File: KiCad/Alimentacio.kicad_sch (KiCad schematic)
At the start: 7 parts, among them J4 Conn_01x01_Pin, U2 LM2596S-5, U7 LM1117DT-3.3

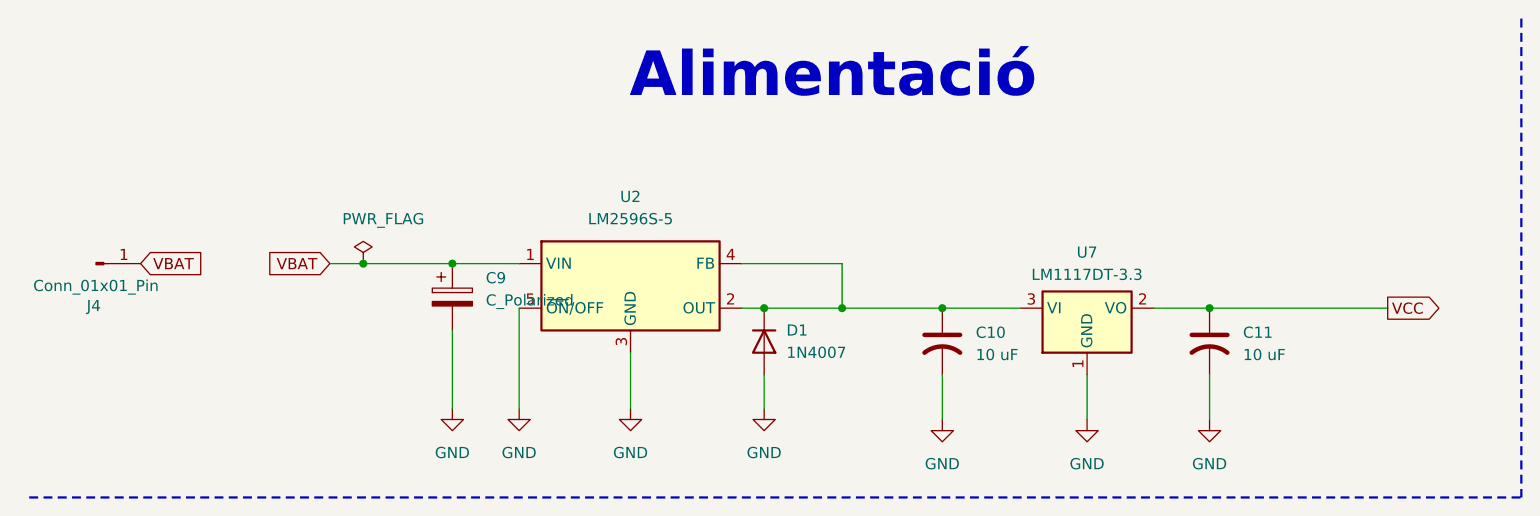
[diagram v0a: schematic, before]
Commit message: Alimentació arreglada
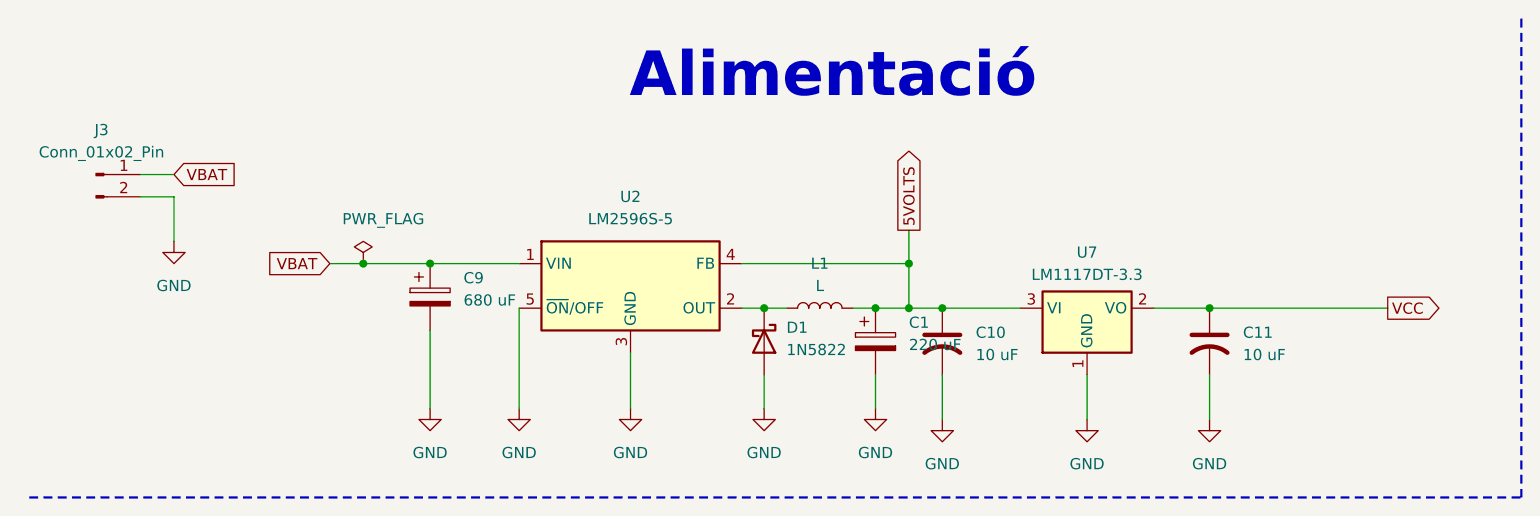
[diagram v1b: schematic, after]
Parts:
- removed D1: 1N4007, Diode_THT:D_DO-41_SOD81_P10.16mm_Horizontal, symbol Diode:1N4007
- removed J4: Conn_01x01_Pin, symbol Connector:Conn_01x01_Pin
- added C1: 220 uF, symbol Device:C_Polarized
- added D1: 1N5822, Diode_THT:D_DO-201AD_P15.24mm_Horizontal, symbol Diode:1N5822
- added J3: Conn_01x02_Pin, symbol Connector:Conn_01x02_Pin
- added L1: L, symbol Device:L
- C9: value C_Polarized -> 680 uF
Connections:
- net GND: now also C1.2, D1.2 (A), J3.2 (Pin_2)
- net VBAT: now also J3.1 (Pin_1)
- net 5VOLTS: now reaches C10.1, U2.4 (FB), U7.3 (VI)
- net 5VOLTS: now also C1.1, L1.2; no longer U2.2 (OUT)
- new net: D1.1 (K), L1.1, U2.2 (OUT)
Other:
- moved on the sheet: C9
